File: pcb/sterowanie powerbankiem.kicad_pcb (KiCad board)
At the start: 2 copper layers, 54.4 x 26 mm, 26 parts, among them J1 USB_A, J2 Conn_01x01_Male, J3 Conn_01x01_Male, Q1 IRLML2060, SW1 SW_DIP_x01, U1 L78L33_SO8, U2 ATtiny13-20SSU

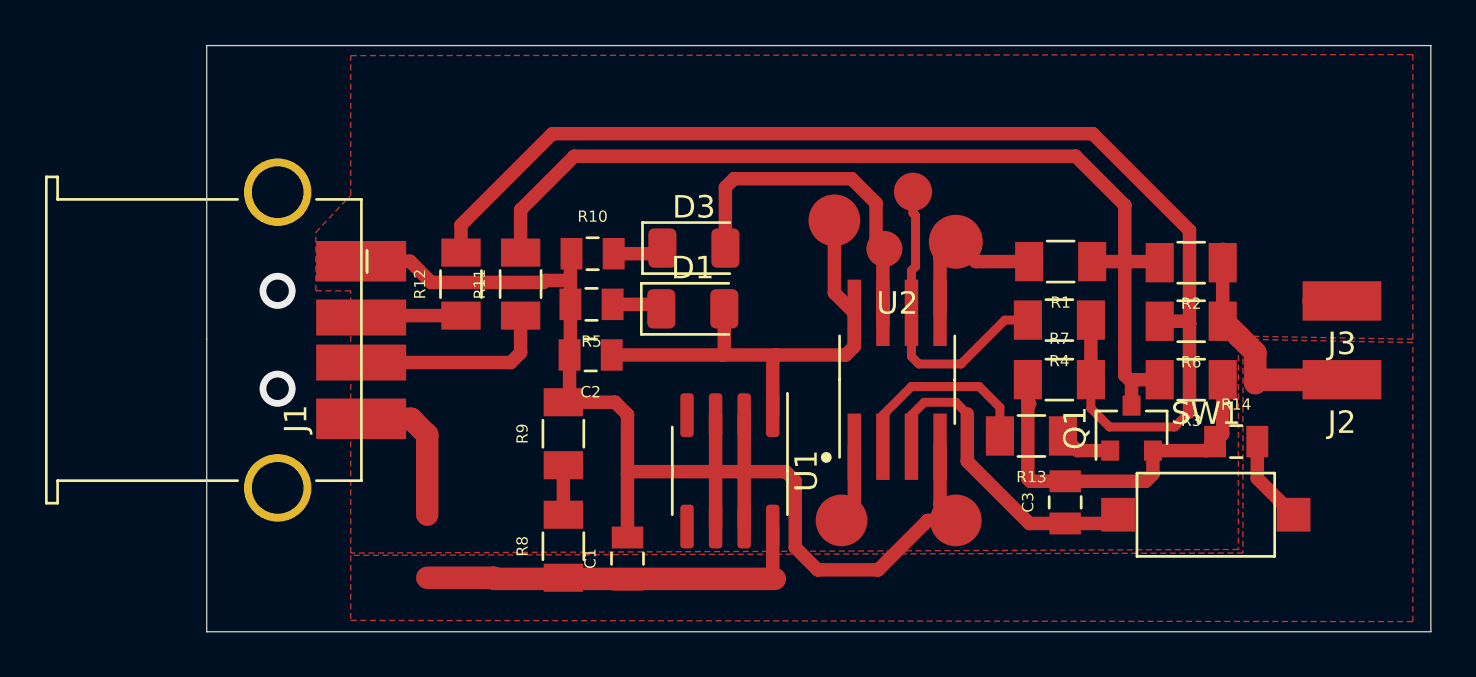
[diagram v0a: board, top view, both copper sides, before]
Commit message: Wersja 1.2
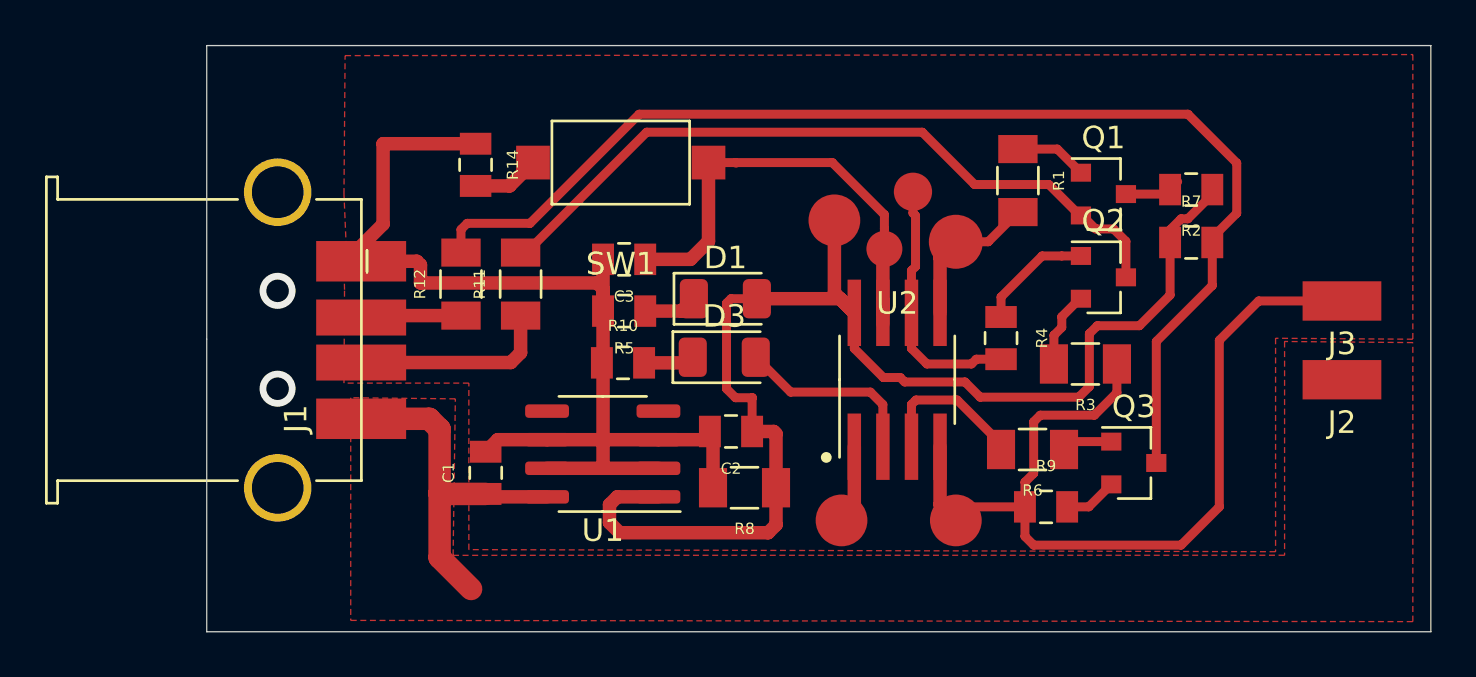
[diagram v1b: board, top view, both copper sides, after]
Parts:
- removed R13: 1K, EKOLED-Elementy pasywne:R_1206
- added Q2: IRLML2060, Package_TO_SOT_SMD:SOT-23, F.Cu at (75.3, 69.3)
- added Q3: IRLML2060, Package_TO_SOT_SMD:SOT-23, F.Cu at (76.7, 77.6)
- R1: value 470R -> 1K
- R2: footprint EKOLED-Elementy pasywne:R_1206 -> EKOLED-Elementy pasywne:R_0805
- R3: value 1K5 -> 2K
- R4: value 470R -> 1K; footprint EKOLED-Elementy pasywne:R_1206 -> EKOLED-Elementy pasywne:R_0805
- R5: value 50R -> 1K
- R6: value 10K -> 1K
- R7: value 1K5 -> 10K; footprint EKOLED-Elementy pasywne:R_1206 -> EKOLED-Elementy pasywne:R_0805
- R8: value 150R -> 100R
- R9: value 150R -> 2K; footprint EKOLED-Elementy pasywne:R_1206 -> EKOLED-Elementy pasywne:R_0805
- moved R14 36.0 mm to (47.4, 64.3), turned to 270 degrees
- moved SW1 30.3 mm to (53.9, 64.2), turned to 180 degrees
- moved C3 22.4 mm to (54.0, 68.5), turned to 180 degrees
- moved R9 21.7 mm to (72.8, 79.5), turned to 0 degrees
- moved Q1 10.5 mm to (75.3, 65.7), turned to 0 degrees
- moved R6 9.07 mm to (72.2, 77.0)
- moved R8 8.46 mm to (59.4, 78.7), turned to 180 degrees
- moved R7 8.45 mm to (79.2, 67.8)
- moved C1 7.36 mm to (47.9, 78.0)
- moved C2 7.10 mm to (58.8, 76.2)
- moved U1 5.70 mm to (53.0, 77.2), turned to 180 degrees
- moved D3 5.03 mm to (58.5, 72.9)
- moved R10 5.03 mm to (54.0, 73.2)
- moved R3 4.75 mm to (74.5, 73.2)
- moved R1 4.07 mm to (71.5, 65.0), turned to 270 degrees
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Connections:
- C3 pad 1: PB4 -> PB2
- D3 pad 2: PB2 -> PB3
- Q1 pad 2: GND -> Net-(Q1-Pad2)
- R1 pad 1: Net-(Q1-Pad3) -> Net-(Q1-Pad1)
- R11 pad 2: Net-(Q1-Pad3) -> Net-(Q1-Pad2)
- R12 pad 2: Net-(R12-Pad2) -> Net-(Q3-Pad3)
- R2 pad 1: +12V -> +3V3
- R3 pad 2: Net-(Q1-Pad3) -> Net-(Q2-Pad2)
- R4 pad 1: Net-(R12-Pad2) -> Net-(Q2-Pad1)
- R6 pad 1: +12V -> Net-(Q3-Pad1)
- R6 pad 2: Net-(R12-Pad2) -> PB4
- R7 pad 1: GND -> +3V3
- R7 pad 2: Net-(R12-Pad2) -> Net-(Q3-Pad3)
- R8 pad 1: +12V -> +3V3
- R8 pad 2: Net-(R8-Pad2) -> GND
- R9 pad 1: Net-(R8-Pad2) -> GND
- R9 pad 2: GND -> Net-(Q3-Pad2)
- SW1 pad 1: PB4 -> PB2
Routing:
- net Net-(R12-Pad2): track 55.4 -> 0.00 mm
- net Net-(Q3-Pad3): track 0.00 -> 53.3 mm
- net Net-(Q1-Pad3): track 44.1 -> 2.12 mm
- net +3V3: track 21.7 -> 58.8 mm
- net Net-(Q1-Pad2): track 0.00 -> 32.7 mm
- net +12V: track 36.1 -> 17.2 mm
- net GND: track 78.7 -> 95.1 mm
- net PB4: track 14.2 -> 7.00 mm
- net Net-(Q2-Pad1): track 0.00 -> 5.19 mm
- net PB2: track 16.1 -> 20.9 mm
- net Net-(Q2-Pad2): track 0.00 -> 3.43 mm
- net Net-(Q3-Pad2): track 0.00 -> 2.38 mm
- net Net-(Q3-Pad1): track 0.00 -> 2.24 mm
- net Net-(R8-Pad2): track 2.20 -> 0.00 mm
- net PB1: track 13.6 -> 11.4 mm
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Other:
- net class Default: clearance 0.3 -> 0.4
- rule trace_clearance: 0.3 -> 0.4
